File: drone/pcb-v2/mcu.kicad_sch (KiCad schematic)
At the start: 26 parts, among them J3 Conn_01x02_Pin, SW3 SW_Push, SW4 SW_SPDT, U4 TLV1117LV33DCYR, U5 STM32F103C8Tx, U6 W25Q128JVS, Y1 Crystal

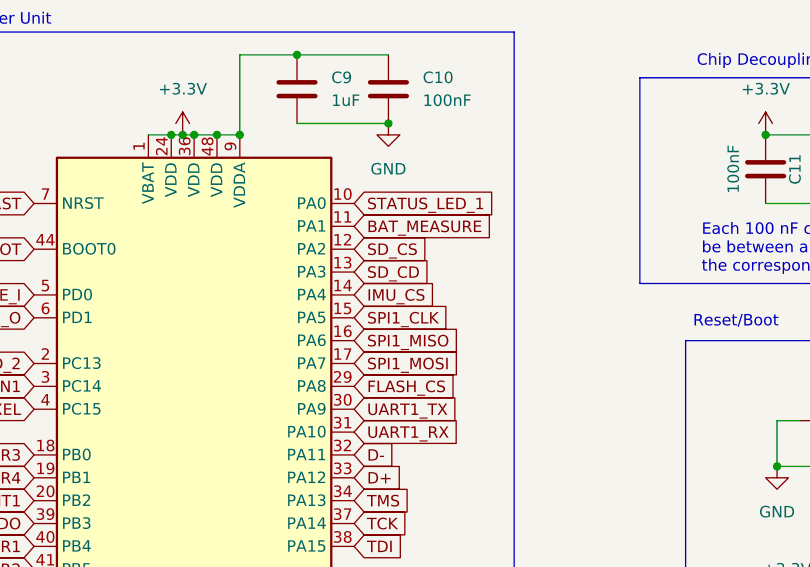
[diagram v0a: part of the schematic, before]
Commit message: [pcb] drc fixes
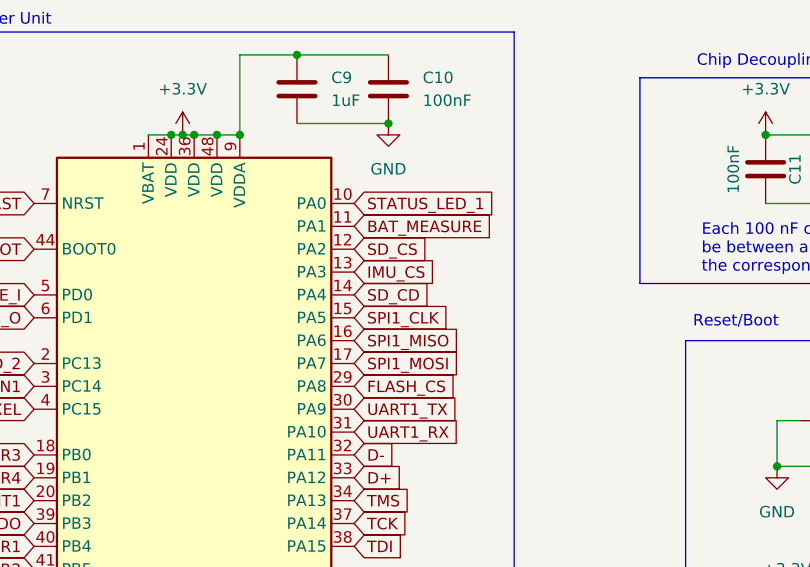
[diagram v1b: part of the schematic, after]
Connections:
- net IMU_CS: now also U5.13 (PA3); no longer U5.14 (PA4)
- net SD_CD: now also U5.14 (PA4); no longer U5.13 (PA3)
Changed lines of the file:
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@@
+		)
+	)
+	(global_label "IMU_CS"
+		(shape input)
+		(at 67.31 41.91 0)
+		(fields_autoplaced yes)
+		(effects
+			(font
+				(size 1.27 1.27)
+			)
+			(justify left)
+		)
+		(property "Intersheetrefs" "${INTERSHEET_REFS}"
+			(at 77.129 41.91 0)
+			(effects
+				(font
+					(size 1.27 1.27)
+				)
+				(justify left)
+				(hide yes)
+			)
 		)
 	)
@@
 		)
 	)
+	(global_label "SD_CD"
+		(shape input)
+		(at 67.31 44.45 0)
+		(fields_autoplaced yes)
+		(effects
+			(font
+				(size 1.27 1.27)
+			)
+			(justify left)
+		)
+		(property "Intersheetrefs" "${INTERSHEET_REFS}"
+			(at 76.2823 44.45 0)
+			(effects
+				(font
+					(size 1.27 1.27)
+				)
+				(justify left)
+				(hide yes)
+			)
+		)
+	)
 	(global_label "RST"
 		(shape input)
@@
 		)
 	)
-	(global_label "IMU_CS"
-		(shape input)
-		(at 67.31 44.45 0)
-		(fields_autoplaced yes)
-		(effects
-			(font
-				(size 1.27 1.27)
-			)
-			(justify left)
-		)
-		(property "Intersheetrefs" "${INTERSHEET_REFS}"
-			(at 77.129 44.45 0)
-			(effects
-				(font
-					(size 1.27 1.27)
-				)
-				(justify left)
-				(hide yes)
-			)
-		)
-	)
 	(global_label "SPI2_MOSI"
 		(shape input)
@@
 			(effects
 				(font
-					(size 1.27 1.27)
-				)
-				(justify left)
-				(hide yes)
-			)
-		)
-	)
-	(global_label "SD_CD"
-		(shape input)
-		(at 67.31 41.91 0)
-		(fields_autoplaced yes)
-		(effects
-			(font
-				(size 1.27 1.27)
-			)
-			(justify left)
-		)
-		(property "Intersheetrefs" "${INTERSHEET_REFS}"
-			(at 76.2823 41.91 0)
-			(effects
-				(font
